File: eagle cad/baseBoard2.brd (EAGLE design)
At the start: 100 x 69.5 mm, 75 parts

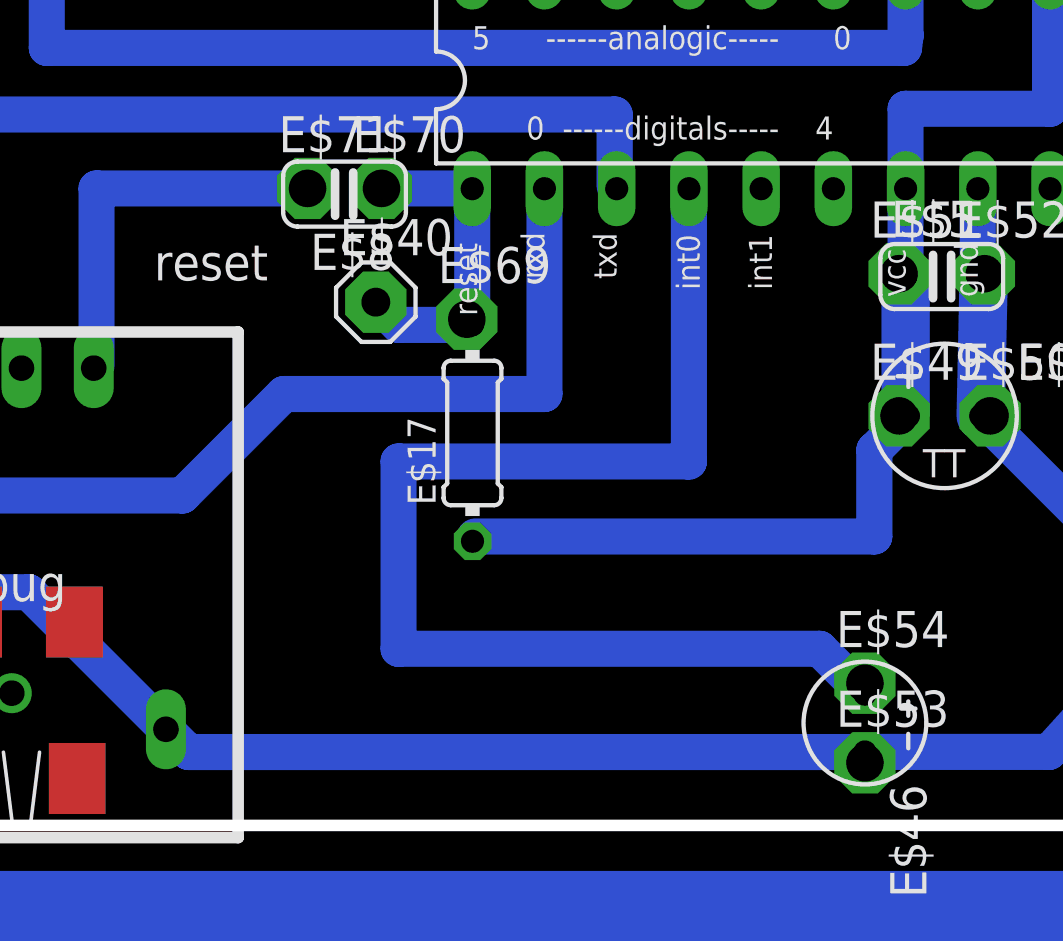
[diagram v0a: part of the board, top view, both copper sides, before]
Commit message: .
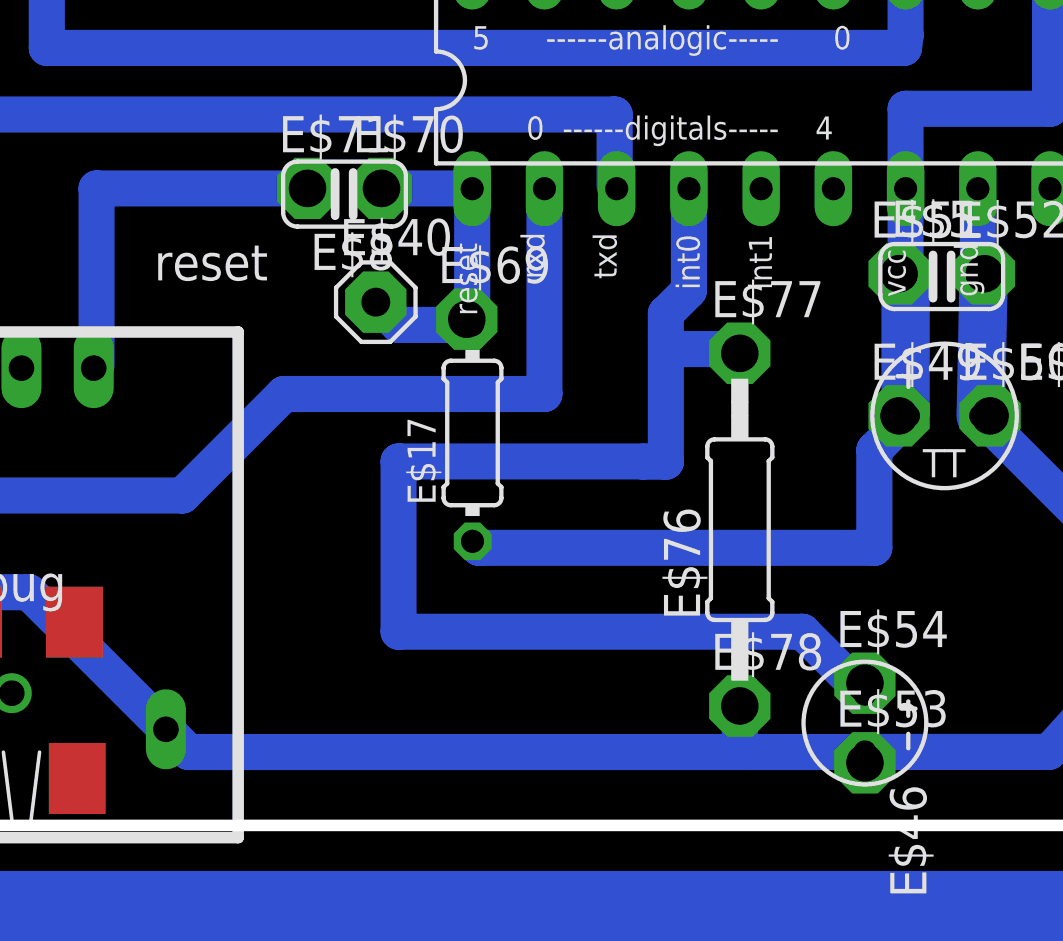
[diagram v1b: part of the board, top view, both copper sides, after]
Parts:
- added E$76: 100K, ref-packages:0207/12
- added E$77, E$78: (no value), testpad:P1-13
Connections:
- net GND: now also E$76.1
- net S$22: now also E$76.2
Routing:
- net S$22: track 43.5 -> 45.4 mm
- net GND: track 274.2 -> 275.8 mm
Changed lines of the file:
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@@
 <?xml version="1.0" encoding="utf-8"?>
 <!DOCTYPE eagle SYSTEM "eagle.dtd">
-<eagle version="8.2.2">
+<eagle version="9.6.2">
 <drawing>
 <settings>
 <setting alwaysvectorfont="no"/>
+<setting keepoldvectorfont="yes"/>
 <setting verticaltext="up"/>
 </settings>
-<grid distance="0.2" unitdist="mm" unit="mm" style="lines" multiple="1" display="yes" altdistance="0.003125" altunitdist="mic" altunit="mm"/>
+<grid distance="0.4" unitdist="mm" unit="mm" style="lines" multiple="1" display="yes" altdistance="0.003125" altunitdist="mic" altunit="mm"/>
 <layers>
 <layer number="1" name="Top" color="4" fill="1" visible="yes" active="yes"/>
@@
 <layer number="17" name="Pads" color="2" fill="1" visible="yes" active="yes"/>
 <layer number="18" name="Vias" color="2" fill="1" visible="yes" active="yes"/>
-<layer number="19" name="Unrouted" color="6" fill="1" visible="no" active="yes"/>
+<layer number="19" name="Unrouted" color="6" fill="1" visible="yes" active="yes"/>
 <layer number="20" name="Dimension" color="15" fill="1" visible="yes" active="yes"/>
-<layer number="21" name="tPlace" color="7" fill="1" visible="no" active="yes"/>
+<layer number="21" name="tPlace" color="7" fill="1" visible="yes" active="yes"/>
 <layer number="22" name="bPlace" color="7" fill="1" visible="no" active="yes"/>
-<layer number="23" name="tOrigins" color="15" fill="1" visible="no" active="yes"/>
-<layer number="24" name="bOrigins" color="15" fill="1" visible="no" active="yes"/>
+<layer number="23" name="tOrigins" color="15" fill="1" visible="yes" active="yes"/>
+<layer number="24" name="bOrigins" color="15" fill="1" visible="yes" active="yes"/>
 <layer number="25" name="tNames" color="7" fill="1" visible="no" active="yes"/>
 <layer number="26" name="bNames" color="7" fill="1" visible="no" active="yes"/>
-<layer number="27" name="tValues" color="7" fill="1" visible="no" active="yes"/>
+<layer number="27" name="tValues" color="7" fill="1" visible="yes" active="yes"/>
 <layer number="28" name="bValues" color="7" fill="1" visible="no" active="yes"/>
 <layer number="29" name="tStop" color="7" fill="3" visible="no" active="yes"/>
@@
 <param name="dpMaxLengthDifference" value="10mm"/>
 <param name="dpGapFactor" value="2.5"/>
-<param name="checkGrid" value="0"/>
 <param name="checkAngle" value="0"/>
 <param name="checkFont" value="1"/>
 <param name="checkRestrict" value="1"/>
+<param name="checkStop" value="0"/>
+<param name="checkValues" value="0"/>
+<param name="checkNames" value="1"/>
+<param name="checkWireStubs" value="1"/>
+<param name="checkPolygonWidth" value="0"/>
 <param name="useDiameter" value="13"/>
 <param name="maxErrors" value="50"/>
@@
 <attribute name="VALUE" x="89.2" y="22.6" size="0.0254" layer="27"/>
 </element>
+<element name="E$76" library="ref-packages" library_urn="urn:adsk.eagle:library:338" package="0207/12" value="100K" x="40.8" y="10.4" smashed="yes" rot="R90">
+<attribute name="NAME" x="39.403" y="7.225" size="1.27" layer="25" ratio="10" rot="R90"/>
+<attribute name="VALUE" x="41.4858" y="8.114" size="1.27" layer="27" ratio="10" rot="R90"/>
+</element>
+<element name="E$77" library="testpad" library_urn="urn:adsk.eagle:library:385" package="P1-13" value="" x="40.8" y="16.6" smashed="yes">
+<attribute name="NAME" x="39.784" y="17.87" size="1.27" layer="25" ratio="10"/>
+<attribute name="VALUE" x="40.8" y="16.6" size="0.0254" layer="27"/>
+</element>
+<element name="E$78" library="testpad" library_urn="urn:adsk.eagle:library:385" package="P1-13" value="" x="40.8" y="4.2" smashed="yes">
+<attribute name="NAME" x="39.784" y="5.47" size="1.27" layer="25" ratio="10"/>
+<attribute name="VALUE" x="40.8" y="4.2" size="0.0254" layer="27"/>
+</element>
 </elements>
 <signals>
@@
 <wire x1="58.07" y1="5.6" x2="64.302" y2="5.6" width="1.27" layer="16"/>
 <wire x1="20.62" y1="3.38" x2="21.42" y2="2.58" width="1.27" layer="16"/>
-<wire x1="45.09573125" y1="2.58" x2="21.42" y2="2.58" width="1.27" layer="16"/>
+<wire x1="45.09573125" y1="2.58" x2="41.2" y2="2.58" width="1.27" layer="16"/>
+<wire x1="41.2" y1="2.58" x2="21.42" y2="2.58" width="1.27" layer="16"/>
 <wire x1="45.09573125" y1="2.58" x2="45.13573125" y2="2.54" width="1.27" layer="16"/>
 <wire x1="45.2" y1="2.584" x2="51.6751625" y2="2.584" width="1.27" layer="16"/>
@@
 <wire x1="49.17" y1="19.3" x2="49.37" y2="19.1" width="1.7" layer="16" curve="4.255771"/>
 <wire x1="49.37" y1="19.1" x2="49.27" y2="14.4" width="1.7" layer="16"/>
-<wire x1="74.58" y1="5.73" x2="80.5" y2="16.05" width="0" layer="19" extent="16-16"/>
-<wire x1="64.302" y1="5.6" x2="63" y2="5.55" width="0" layer="19" extent="16-16"/>
+<contactref element="E$76" pad="1"/>
+<wire x1="40.8" y1="4.05" x2="40.8" y2="2.98" width="1.27" layer="16"/>
+<wire x1="40.8" y1="2.98" x2="41.2" y2="2.58" width="0.7" layer="16"/>
+<wire x1="74.58" y1="5.73" x2="80.5" y2="16.05" width="0" layer="19" extent="1-1"/>
+<wire x1="64.42" y1="5.73" x2="63" y2="5.55" width="0" layer="19" extent="16-16"/>
 </signal>
 <signal name="S$5">
@@
 <wire x1="85.9" y1="16.19" x2="85.9" y2="22.63" width="1.27" layer="16"/>
 <contactref element="E$20" pad="+"/>
-<wire x1="45.53" y1="10.16" x2="31.49" y2="10.16" width="1.27" layer="16"/>
+<wire x1="45.53" y1="9.76" x2="31.63" y2="9.76" width="1.27" layer="16"/>
+<wire x1="31.4" y1="9.99" x2="31.63" y2="9.76" width="1.27" layer="16"/>
 <contactref element="E$17" pad="1"/>
-<wire x1="31.49" y1="10.16" x2="31.4" y2="9.99" width="0.7" layer="16"/>
 <wire x1="46.63" y1="19.3" x2="46.63" y2="14.5" width="1.7" layer="16"/>
 <wire x1="46.63" y1="14.5" x2="46.73" y2="14.4" width="0.8128" layer="16"/>
 <wire x1="46.73" y1="14.4" x2="45.53" y2="13.2" width="1.27" layer="16"/>
-<wire x1="45.53" y1="13.2" x2="45.53" y2="10.16" width="1.27" layer="16"/>
+<wire x1="45.53" y1="13.2" x2="45.53" y2="9.76" width="1.27" layer="16"/>
 <wire x1="51.37" y1="39.6" x2="50.97" y2="39.2" width="1.27" layer="16"/>
 <wire x1="50.97" y1="39.2" x2="49.37" y2="37.6" width="1.27" layer="16"/>
@@
 <contactref element="E$46" pad="+"/>
 <contactref element="E$19" pad="4"/>
-<wire x1="45.2" y1="4.616" x2="43.606" y2="6.21" width="1.27" layer="16"/>
-<wire x1="43.606" y1="6.21" x2="28.8" y2="6.21" width="1.27" layer="16"/>
-<wire x1="39.00875" y1="12.8" x2="28.8" y2="12.8" width="1.27" layer="16"/>
-<wire x1="28.8" y1="12.8" x2="28.8" y2="6.21" width="1.27" layer="16"/>
-<wire x1="39.00875" y1="12.8" x2="39.01" y2="12.79" width="0.7" layer="16"/>
-<wire x1="39.01" y1="12.79" x2="39.01" y2="22.39" width="1.27" layer="16"/>
+<wire x1="45.2" y1="4.616" x2="43.006" y2="6.81" width="1.27" layer="16"/>
+<wire x1="43.006" y1="6.81" x2="28.8" y2="6.81" width="1.27" layer="16"/>
+<wire x1="37.40875" y1="12.8" x2="28.8" y2="12.8" width="1.27" layer="16"/>
+<wire x1="28.8" y1="12.8" x2="28.8" y2="6.81" width="1.27" layer="16"/>
+<wire x1="37.40875" y1="12.8" x2="37.41" y2="12.79" width="0.7" layer="16"/>
+<wire x1="37.41" y1="12.79" x2="38.2" y2="12.79" width="1.27" layer="16"/>
+<wire x1="38.2" y1="12.79" x2="38.2" y2="17.2" width="1.27" layer="16"/>
+<wire x1="38.2" y1="17.2" x2="38.2" y2="18" width="1.27" layer="16"/>
+<wire x1="38.2" y1="18" x2="39.01" y2="18.81" width="1.27" layer="16"/>
+<wire x1="39.01" y1="18.81" x2="39.01" y2="22.39" width="1.27" layer="16"/>
+<contactref element="E$76" pad="2"/>
+<wire x1="40.8" y1="16.75" x2="38.65" y2="16.75" width="1.27" layer="16"/>
+<wire x1="38.65" y1="16.75" x2="38.2" y2="17.2" width="0.7" layer="16"/>
 </signal>
 <signal name="S$10">
@@
 </signal>
 </signals>
+<mfgpreviewcolors>
+<mfgpreviewcolor name="soldermaskcolor" color="0xC8008000"/>
+<mfgpreviewcolor name="silkscreencolor" color="0xFFFEFEFE"/>
+<mfgpreviewcolor name="backgroundcolor" color="0xFF282828"/>
+<mfgpreviewcolor name="coppercolor" color="0xFFFFBF00"/>
+<mfgpreviewcolor name="substratecolor" color="0xFF786E46"/>
+</mfgpreviewcolors>
 </board>
 </drawing>
 <compatibility>
 <note version="8.2" severity="warning">
-Since Version 8.2, Eagle supports online libraries. The ids
+Since Version 8.2, EAGLE supports online libraries. The ids
 of those online libraries will not be understood (or retained)
 with this version.
